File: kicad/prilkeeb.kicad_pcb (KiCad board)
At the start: 2 copper layers, 176.1 x 130.6 mm, 77 parts, among them SW1 SW_SPDT, U2 Nice_Nano_V2

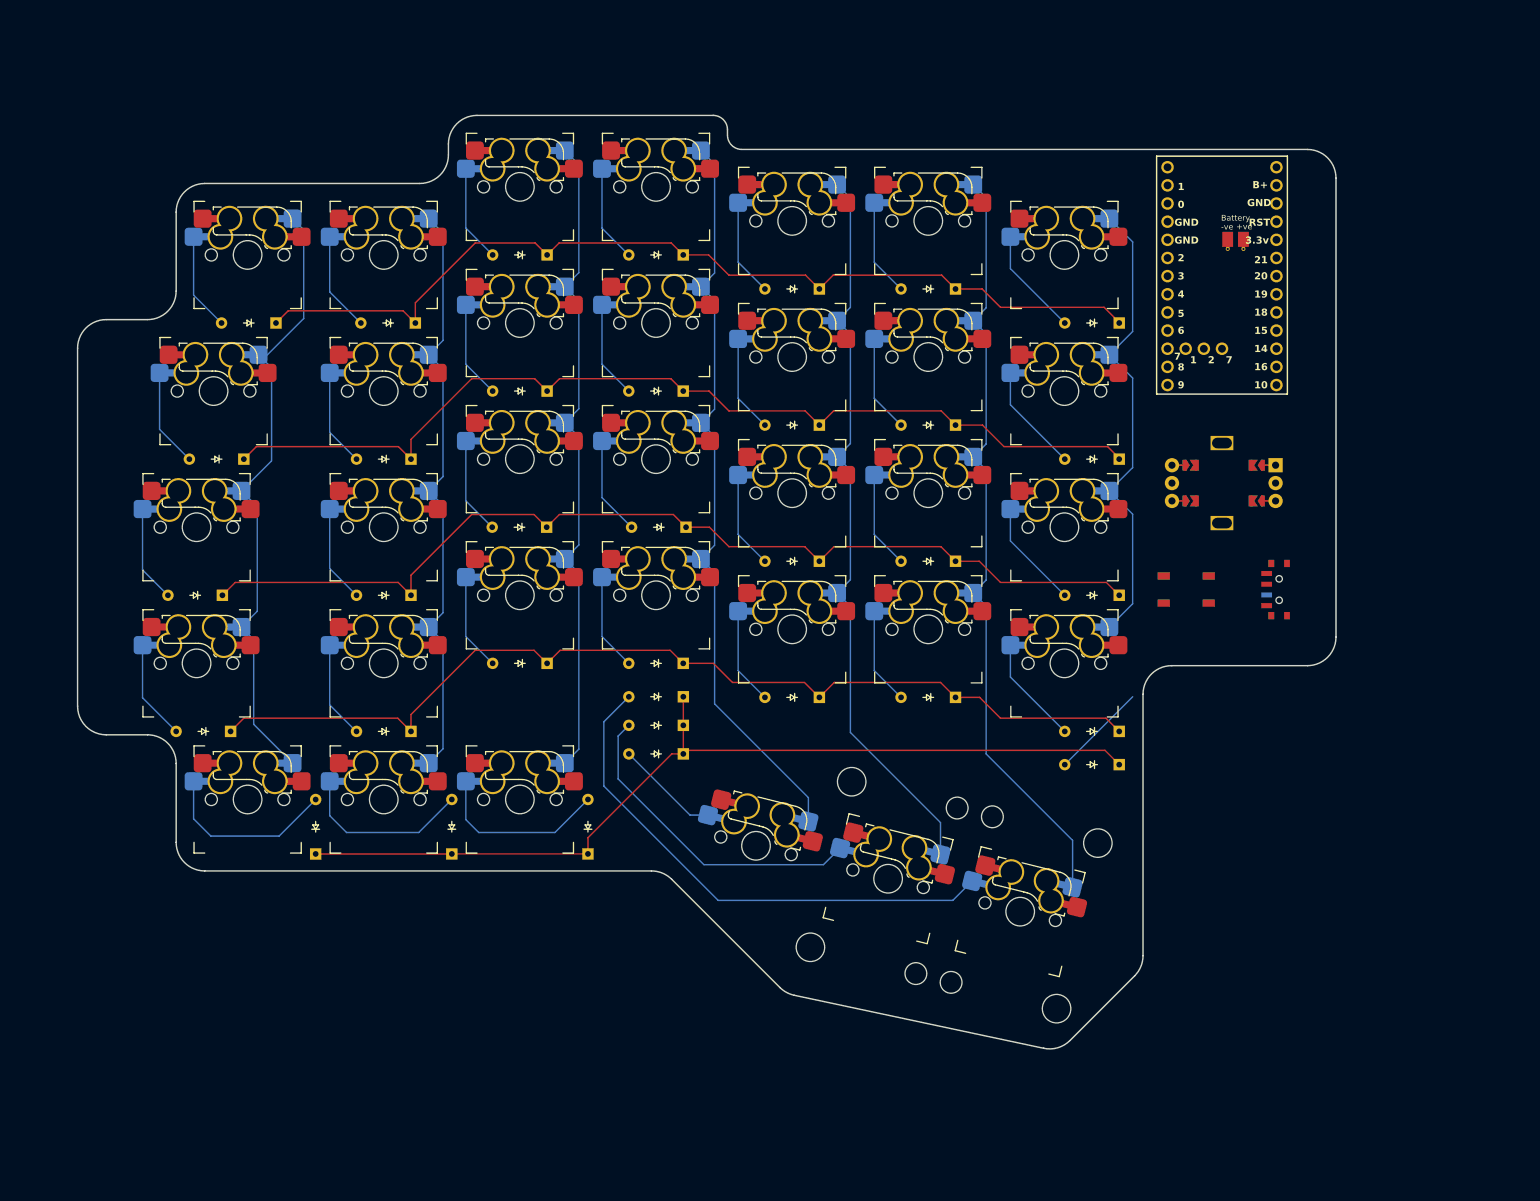
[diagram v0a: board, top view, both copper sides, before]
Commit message: Routing
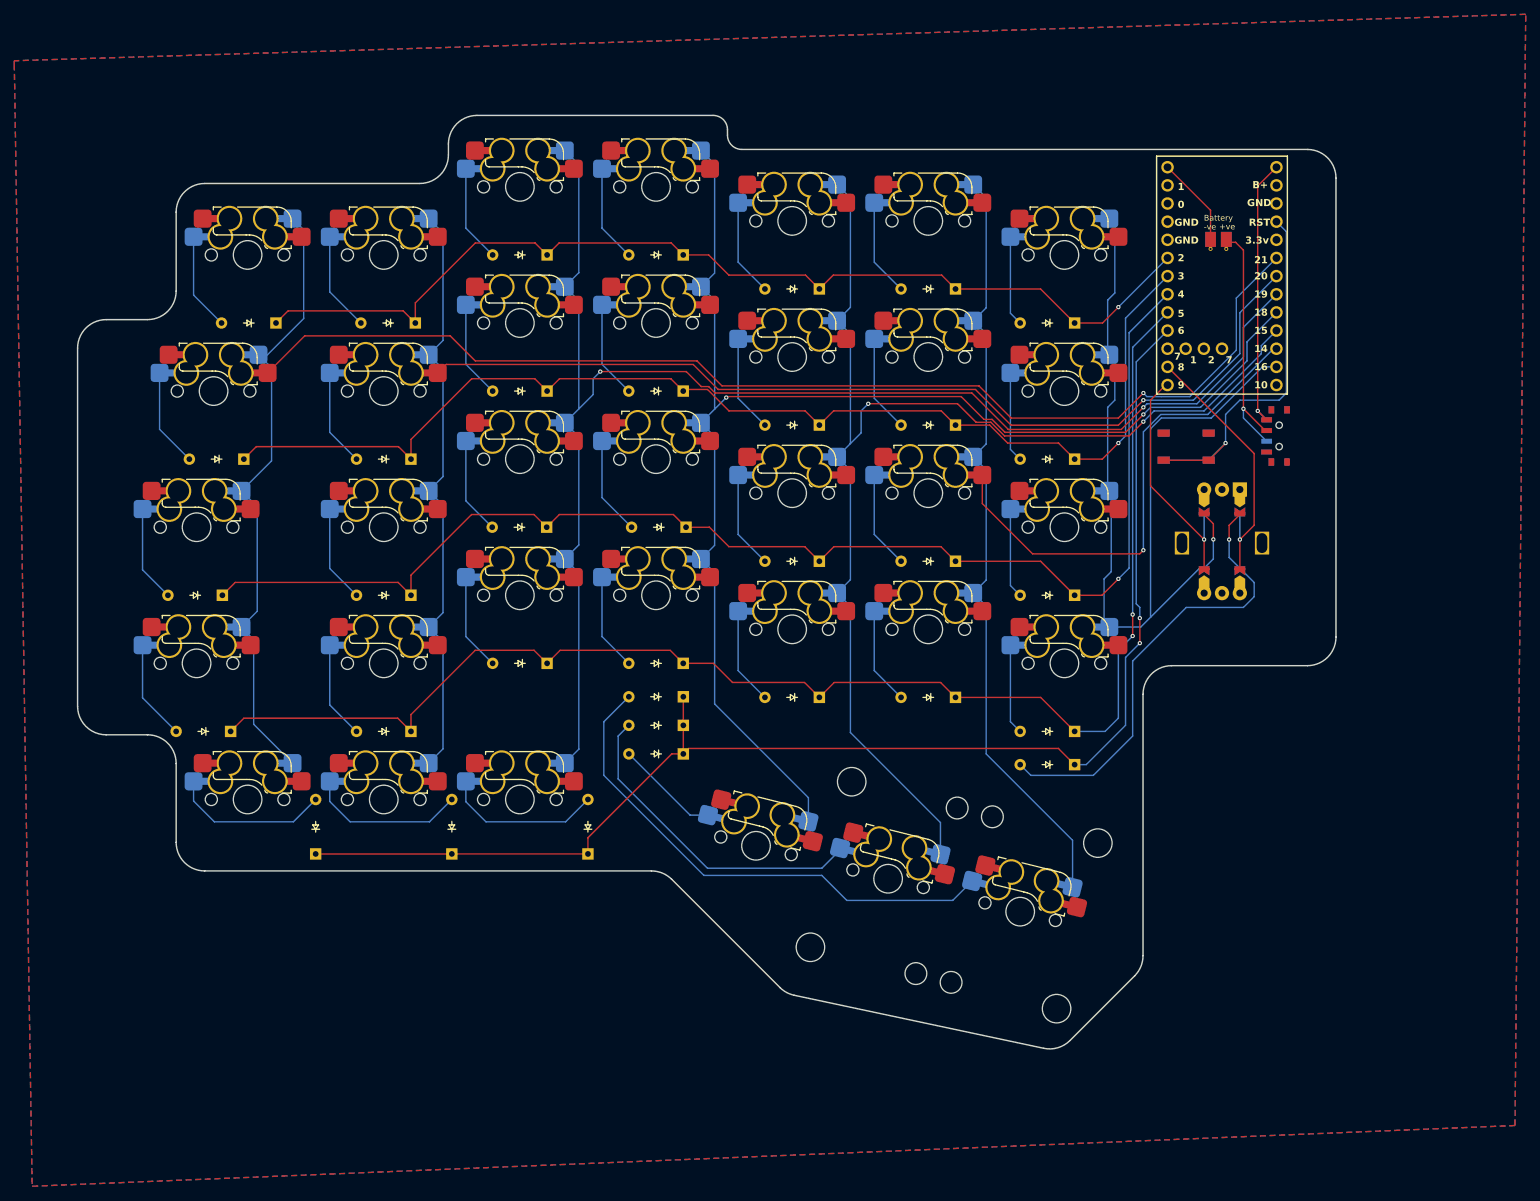
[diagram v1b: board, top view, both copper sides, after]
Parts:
- ROT1: moved to F.Cu
- moved SW1 21.5 mm to (201.5, 92.0)
- moved RST_SW1 20.0 mm to (188.5, 93.5)
- moved RST_SW2 20.0 mm to (188.5, 93.5)
- moved ROT1 8.40 mm to (193.5, 107.0), turned to -90 degrees
- moved D14 6.24 mm to (172.9, 95.2)
- moved D21 6.24 mm to (172.9, 114.3)
- moved D28 6.24 mm to (172.9, 133.3)
- moved D7 6.24 mm to (172.9, 76.2)
- moved DROTARY1 6.24 mm to (172.9, 138.0)
- moved BT1 2.40 mm to (193.0, 64.5)
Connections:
- ROT1 pad C: unconnected-(ROT1-PadC) -> GND
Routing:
- net Col_1: track 87.5 -> 249.5 mm, vias 0 -> 1
- net Col_2: track 82.9 -> 216.2 mm, vias 0 -> 1
- net Col_3: track 92.2 -> 206.9 mm, vias 0 -> 2
- net Col_4: track 104.9 -> 194.8 mm, vias 0 -> 2
- net Col_5: track 104.3 -> 176.7 mm, vias 0 -> 2
- net Col_6: track 108.6 -> 178.2 mm, vias 0 -> 1
- net Col_7: track 65.3 -> 132.5 mm, vias 0 -> 1
- net Row_5: track 128.6 -> 190.1 mm, vias 0 -> 2
- net Row_4: track 139.9 -> 200.2 mm, vias 0 -> 2
- net RST: track 0.00 -> 57.6 mm, vias 0 -> 1
- net Net-(DROTARY1-A): track 13.4 -> 63.4 mm, vias 0 -> 1
- net Row_3: track 141.2 -> 184.7 mm, vias 0 -> 1
- net B+: track 0.00 -> 38.7 mm, vias 0 -> 1
- net RotaryA: track 0.00 -> 37.5 mm, vias 0 -> 1
- net Net-(BT1-+): track 0.00 -> 35.4 mm, vias 0 -> 1
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- added copper zone on B.Cu, net GND
- added copper zone on F.Cu, net GND
